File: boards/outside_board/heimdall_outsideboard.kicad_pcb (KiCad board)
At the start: 2 copper layers, 6 parts, among them J1 Conn_01x09, J2 Conn_01x06

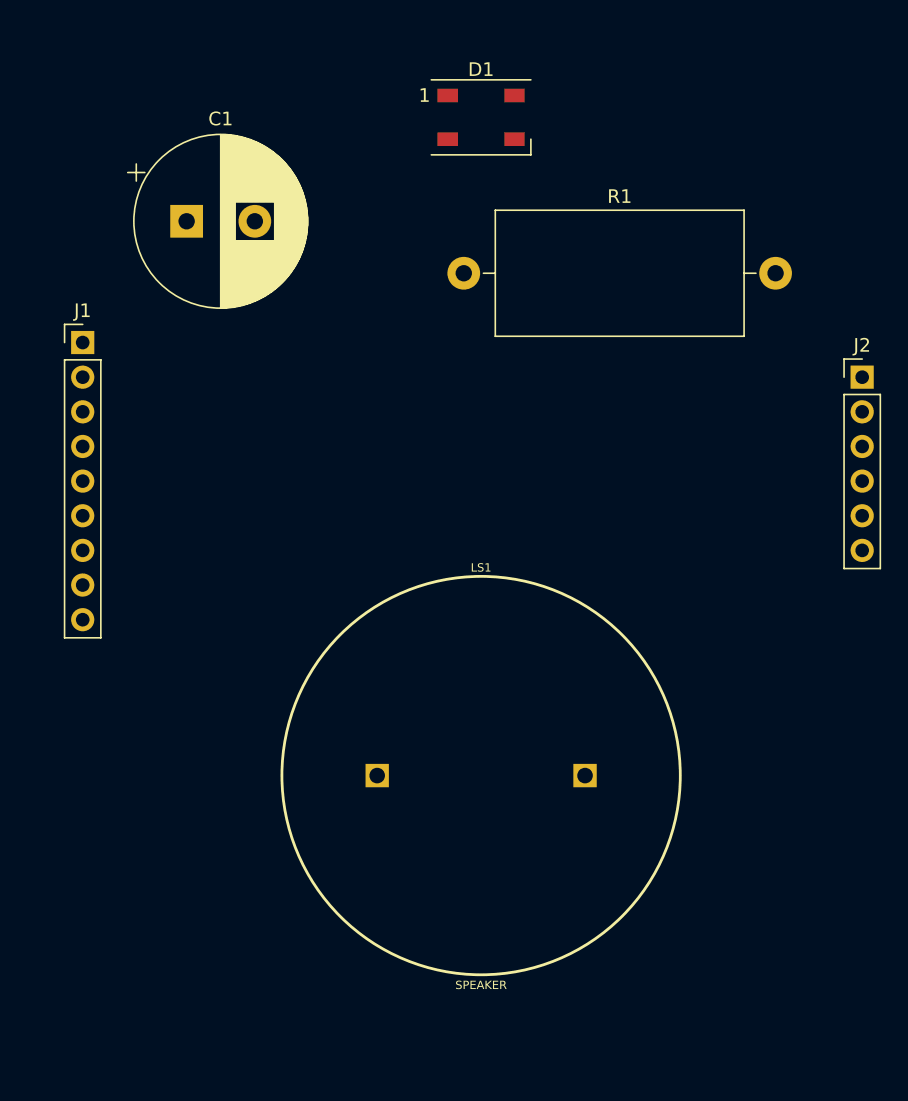
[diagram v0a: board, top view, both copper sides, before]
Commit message: More outside board PCB layout.
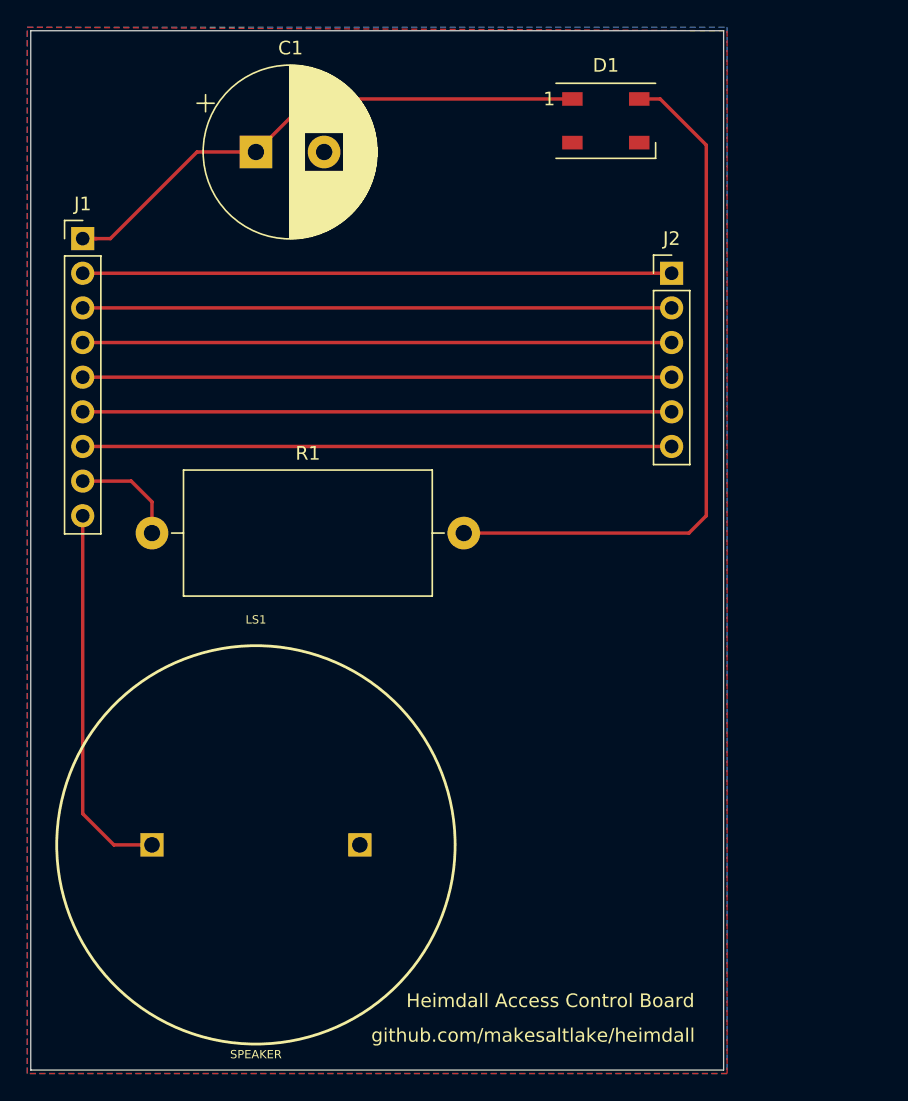
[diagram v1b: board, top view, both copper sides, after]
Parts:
- moved R1 29.8 mm to (59.7, 113.0)
- moved LS1 17.3 mm to (67.3, 135.9)
- moved J2 15.9 mm to (97.8, 94.0)
- moved D1 9.15 mm to (93.0, 82.8)
- moved J1 7.62 mm to (54.6, 91.4)
- moved C1 7.18 mm to (67.3, 85.1)
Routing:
- net Net-(D1-Pad4): track 0.00 -> 51.8 mm
- net /SCK: track 0.00 -> 43.2 mm
- net /MOSI: track 0.00 -> 43.2 mm
- net /MISO: track 0.00 -> 43.2 mm
- net /GND: track 0.00 -> 43.2 mm
- net /CS: track 0.00 -> 43.2 mm
- net /+3V3: track 0.00 -> 43.2 mm
- net /+5V: track 0.00 -> 41.2 mm
- net /Buzzer: track 0.00 -> 27.9 mm
- net /LED: track 0.00 -> 8.00 mm
- added copper zone on B.Cu, net /GND
- added copper zone on F.Cu, net /GND
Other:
- board outline added: 50.8 x 76.2 mm
- board text added: "Heimdall Access Control Board"
- board text added: "github.com/makesaltlake/heimdall"
